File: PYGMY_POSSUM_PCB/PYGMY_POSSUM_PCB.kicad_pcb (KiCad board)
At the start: 2 copper layers, 63 x 58 mm, 27 parts, among them J2 AudioJack, Q1 2N7002, Q2 AO3401A, Q3 AO3401A, Q4 2N7002, Q5 2N7002, Q6 2N7002, U2 PS2501-1, U3 CH340G, U4 AMS1117-3.3, U5 PIC16F18344-SO, Y1 12MHz

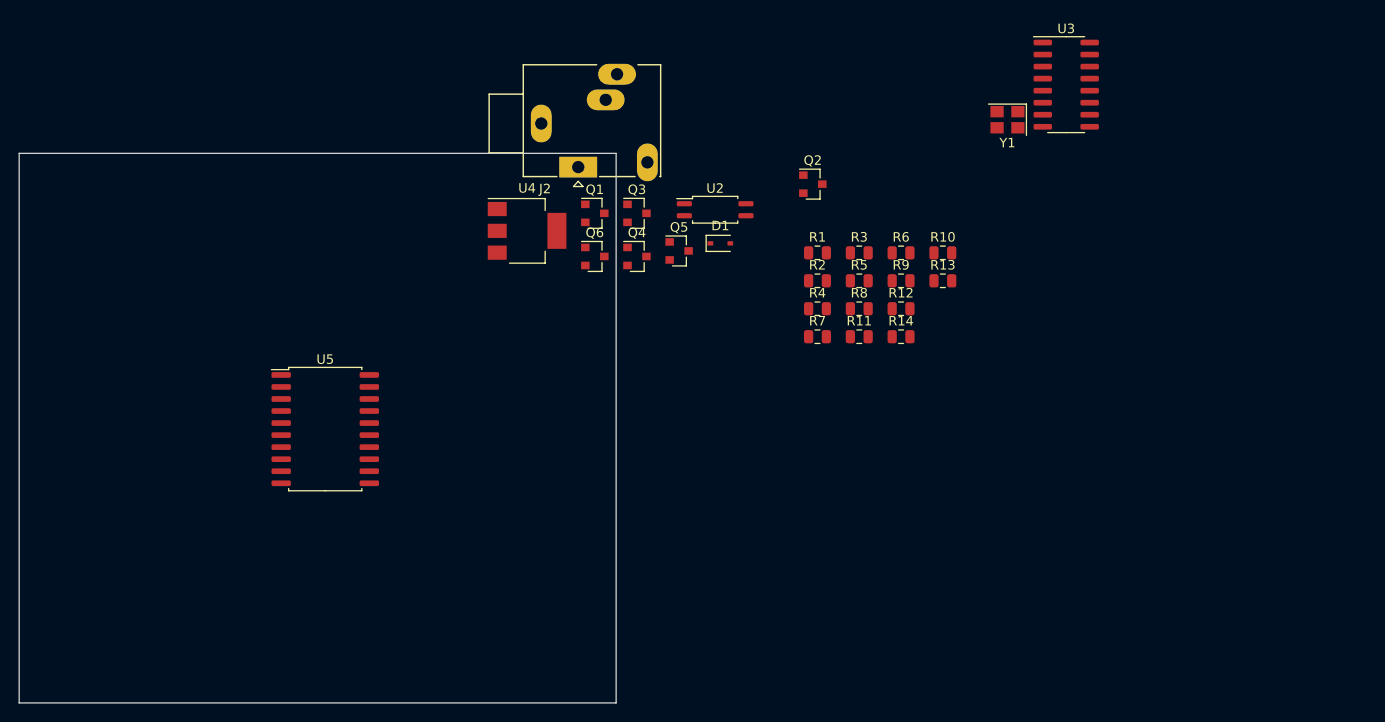
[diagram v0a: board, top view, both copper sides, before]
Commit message: Updates
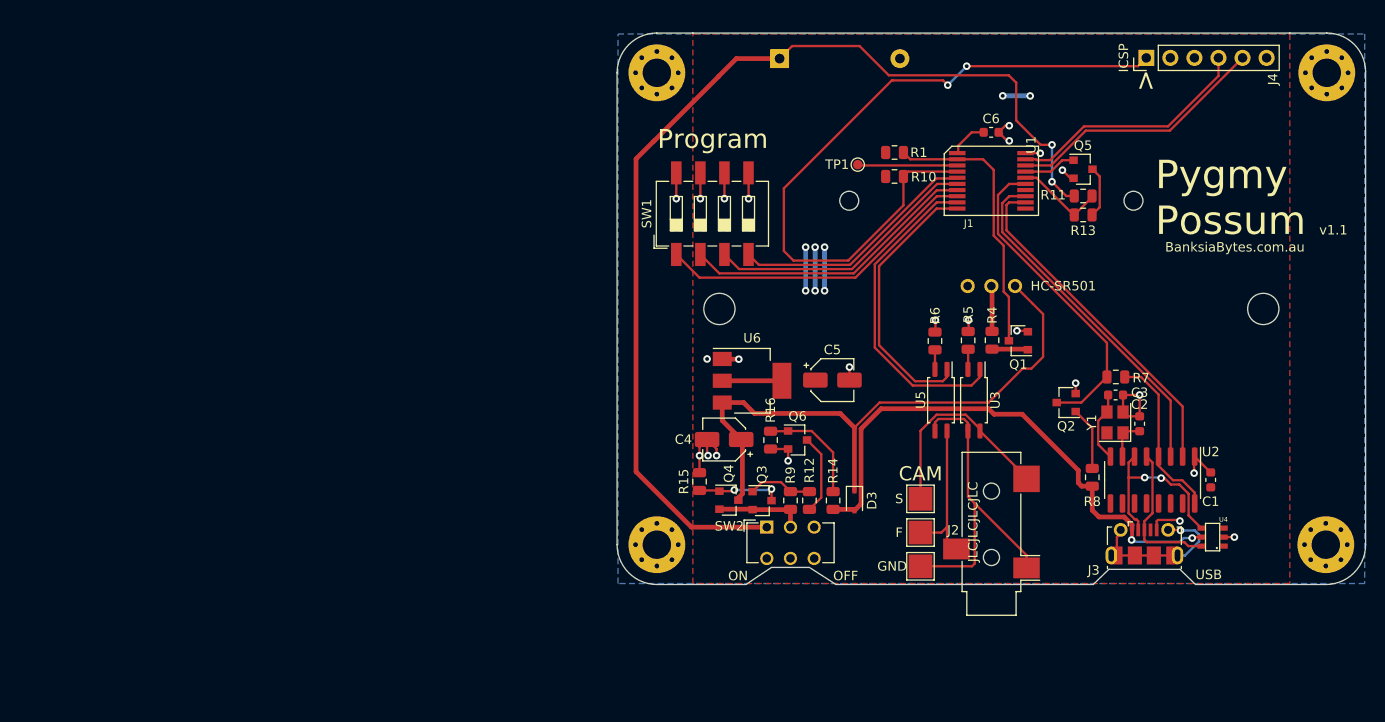
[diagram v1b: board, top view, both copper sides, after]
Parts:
- removed the Q6 at (126.8, 97.4)
- removed the R1 at (150.2, 97.0)
- removed the R10 at (163.5, 97.0)
- removed the R8 at (154.7, 102.9)
- added BT1: 4*AA, BANKSIA_BYTES_FOOTPRINTS:BatteryHolder_Keystone_2462_2xAA, B.Cu at (146.2, 76.5)
- added C1: 0.1uF, Capacitor_SMD:C_0603_1608Metric, F.Cu at (191.8, 121.0)
- added C2: 10pF, Capacitor_SMD:C_0603_1608Metric, F.Cu at (184.2, 115.0)
- added C3: 10pF, Capacitor_SMD:C_0603_1608Metric, F.Cu at (181.7, 112.0)
- added C4: CP10u, Capacitor_SMD:CP_Elec_4x3.9, F.Cu at (140.4, 116.7)
- added C5: CP10u, Capacitor_SMD:CP_Elec_4x3.9, F.Cu at (151.8, 110.4)
- added C6: 0.1uF, Capacitor_SMD:C_0603_1608Metric, F.Cu at (168.6, 84.3)
- added G***: LOGO, BANKSIA_BYTES_FOOTPRINTS:PYGMY_CAMERA, B.Cu at (158.3, 101.5)
- added H1: MountingHole_Pad, MountingHole:MountingHole_3mm_Pad_Via, F.Cu at (204.0, 78.0)
- added H2: MountingHole_Pad, MountingHole:MountingHole_3mm_Pad_Via, F.Cu at (133.3, 78.0)
- added H3: MountingHole_Pad, MountingHole:MountingHole_3mm_Pad_Via, F.Cu at (133.3, 127.8)
- added H4: MountingHole_Pad, MountingHole:MountingHole_3mm_Pad_Via, F.Cu at (203.9, 127.8)
- added J1: HC-SR501, BANKSIA_BYTES_FOOTPRINTS:HC-SR501, F.Cu at (168.6, 90.5)
- added J3: USB_B_Micro, Connector_USB:USB_Micro-B_Molex-105017-0001, F.Cu at (184.8, 127.7)
- added J4: Conn_PIC_ICSP_ICD, Connector_PinHeader_2.54mm:PinHeader_1x06_P2.54mm_Vertical, F.Cu at (184.9, 76.4)
- added Q1: 2N7002, Package_TO_SOT_SMD:SOT-23, F.Cu at (171.4, 106.3)
- added R14: 10K, Resistor_SMD:R_0805_2012Metric, F.Cu at (151.9, 123.1)
- added R4: 1K, Resistor_SMD:R_0805_2012Metric, F.Cu at (168.7, 106.2)
- added R5: 1K, Resistor_SMD:R_0805_2012Metric, F.Cu at (166.2, 106.2)
- added SW1: SW_DIP_x04, Button_Switch_SMD:SW_DIP_SPSTx04_Slide_6.7x11.72mm_W8.61mm_P2.54mm_LowProfile, F.Cu at (139.2, 92.9)
- added SW2: SW_SPST, Button_Switch_THT:SW_CuK_JS202011AQN_DPDT_Angled, F.Cu at (144.9, 126.0)
- added TP1: TestPoint, TestPoint:TestPoint_Pad_D1.0mm, F.Cu at (154.5, 87.7)
- added TP2: S, TestPoint:TestPoint_Pad_2.5x2.5mm, F.Cu at (161.1, 123.0)
- added TP3: F, TestPoint:TestPoint_Pad_2.5x2.5mm, F.Cu at (161.1, 126.5)
- added TP4: GND, TestPoint:TestPoint_Pad_2.5x2.5mm, F.Cu at (161.1, 130.1)
- added U3: PS2501-1, Package_SO:SOIC-4_4.55x2.6mm_P1.27mm, F.Cu at (166.8, 112.5)
- added U4: IP4220CZ6, BANKSIA_BYTES_FOOTPRINTS:SOT457, F.Cu at (191.9, 127.0)
- D3: renamed from D1; value BAT60A -> BAT60B
- J2: footprint Connector_Audio:Jack_3.5mm_Ledino_KB3SPRS_Horizontal -> Connector_Audio:Jack_3.5mm_CUI_SJ-3523-SMT_Horizontal
- U1: renamed from U5; footprint Package_SO:SOIC-20W_7.5x12.8mm_P1.27mm -> BANKSIA_BYTES_FOOTPRINTS:SSOP-20
- moved U1 75.0 mm to (168.6, 89.4), turned to 270 degrees
- moved J2 58.3 mm to (168.6, 126.7), turned to 180 degrees
- moved Q2 47.9 mm to (176.5, 112.8), turned to 180 degrees
- moved Q5 43.5 mm to (178.3, 88.2)
- moved U2 42.7 mm to (185.6, 121.0), turned to 270 degrees
- moved Y1 33.9 mm to (181.7, 114.9), turned to 90 degrees
- moved Q3 33.8 mm to (144.4, 123.2)
- moved R8 32.6 mm to (179.2, 120.7), turned to 270 degrees
- moved R15 32.2 mm to (137.8, 121.1), turned to 90 degrees
- moved Q6 32.1 mm to (148.2, 116.8)
- moved Q4 31.8 mm to (140.9, 123.1)
- moved U5 31.2 mm to (163.3, 112.5), turned to 270 degrees
- moved D3 30.6 mm to (154.2, 123.2), turned to 270 degrees
- moved U6 28.5 mm to (143.3, 110.5)
- moved R11 27.9 mm to (178.3, 91.0), turned to 180 degrees
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- renumbered Q4 to Q2, Q2 to Q3, Q3 to Q4, Q1 to Q6, R13 to R1, R14 to R10, R5 to R12, R12 to R13, R6 to R15, R2 to R16, R3 to R6, R9 to R7, R7 to R8, R4 to R9, U3 to U2, U2 to U5, U4 to U6
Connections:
- net Net-(C1-Pad2) renamed /Xi
- net Net-(C2-Pad2) renamed /Xo
- net PIC_Rx renamed /PIC_Rx
- net PIC_Tx renamed /PIC_Tx
- R1 pad 2: DIN_PIR -> /DIN_PIR
- R11 pad 1: ANIN_BAT_CHECK_VADC -> ANIN_BAT_CHECK
- R13 pad 2: ANIN_BAT_CHECK_VADC -> ANIN_BAT_CHECK
- R6 pad 1: Net-(R3-Pad1) -> Net-(R6-Pad1)
- R6 pad 2: DOUT_CAM -> GND
- U1 pad 10: Net-(U5-Pad10) -> /DOUT_CAM_F
- U1 pad 14: DIN_USB_ON -> Net-(U1-Pad14)
- U1 pad 15: ANIN_BAT_CHECK_VADC -> DIN_USB_ON
- U1 pad 16: DOUT_BAT_CHECK_EN -> ANIN_BAT_CHECK
- U1 pad 17: Net-(U5-Pad17) -> DOUT_BAT_CHECK_EN
- U1 pad 2: DOUT_CAM -> /DIN_PIR
- U1 pad 3: Net-(U5-Pad3) -> /TP_CLK
- U1 pad 5: Net-(SW2-Pad2) -> /DIP1
- U1 pad 6: Net-(SW2-Pad1) -> /DIP2
- U1 pad 7: DIN_PIR -> /DIP3
- U1 pad 8: Net-(SW2-Pad3) -> /DIP4
- U1 pad 9: Net-(SW2-Pad4) -> /DOUT_CAM_S
- U2 pad 5: Net-(J1-Pad3) -> /D+
- U2 pad 6: Net-(J1-Pad2) -> /D-
- U5 pad 1: Net-(R3-Pad1) -> /DOUT_CAM_F
- U5 pad 2: GND -> Net-(R6-Pad1)
- U5 pad 4: Net-(J2-PadT) -> Net-(J2-PadR)
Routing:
- net VBAT: track 0.00 -> 111.6 mm, vias 0 -> 2
- net VPP: track 0.00 -> 75.5 mm, vias 0 -> 2
- net HC-SR501_VCC: track 0.00 -> 65.8 mm
- net VBUS: track 0.00 -> 58.2 mm, vias 0 -> 2
- net GND: track 0.00 -> 48.5 mm, vias 0 -> 23
- net +3V3: track 0.00 -> 44.9 mm, vias 0 -> 8
- net /PIC_Tx: track 0.00 -> 36.8 mm
- net /PIC_Rx: track 0.00 -> 36.3 mm
- net Net-(J2-PadS): track 0.00 -> 35.3 mm
- net /DOUT_CAM_S: track 0.00 -> 35.2 mm
- net /DIP4: track 0.00 -> 34.3 mm
- net DIN_USB_ON: track 0.00 -> 33.7 mm
- net /DIP3: track 0.00 -> 31.7 mm
- net /DIP2: track 0.00 -> 29.0 mm
- net /DIN_PIR: track 0.00 -> 29.0 mm
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- added copper zone on F.Cu, net +3V3
- added copper zone on B.Cu, net GND
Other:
- board size 63 x 58 mm -> 79 x 58.2 mm
- board text added: "BanksiaBytes.com.au"
- board text added: "CAM"
- board text added: "JLCJLCJLCJLC"
- board text added: "OFF"
- board text added: "ON"
- board text added: "Program"
- board text added: "Pygmy Possum"
- board text added: "USB"
- board text added: "v1.1"
